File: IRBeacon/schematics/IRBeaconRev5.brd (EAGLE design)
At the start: 90 x 14.8 mm, 14 parts, among them IC1 LD117AS33TR, SW1 416131160808, X1 53048-06

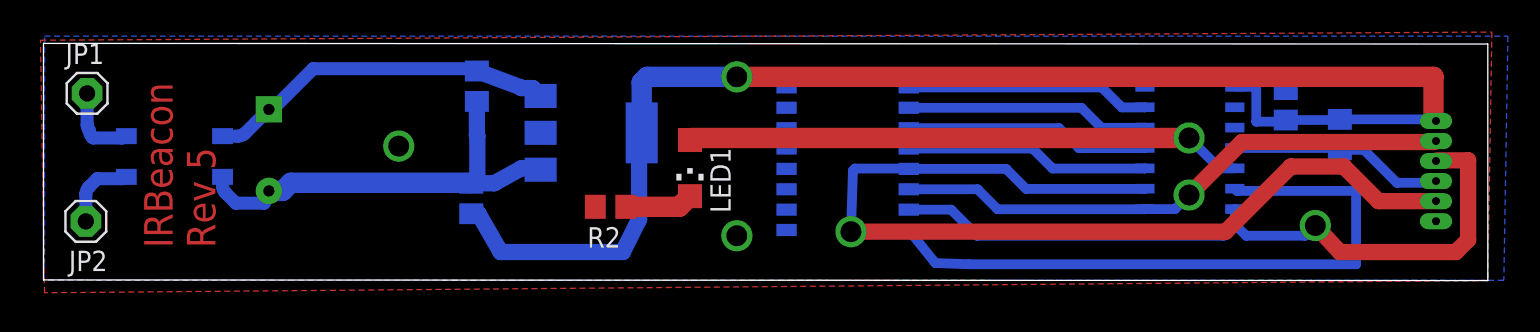
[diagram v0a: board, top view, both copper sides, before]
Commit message: More pinne fix and circuit stuff
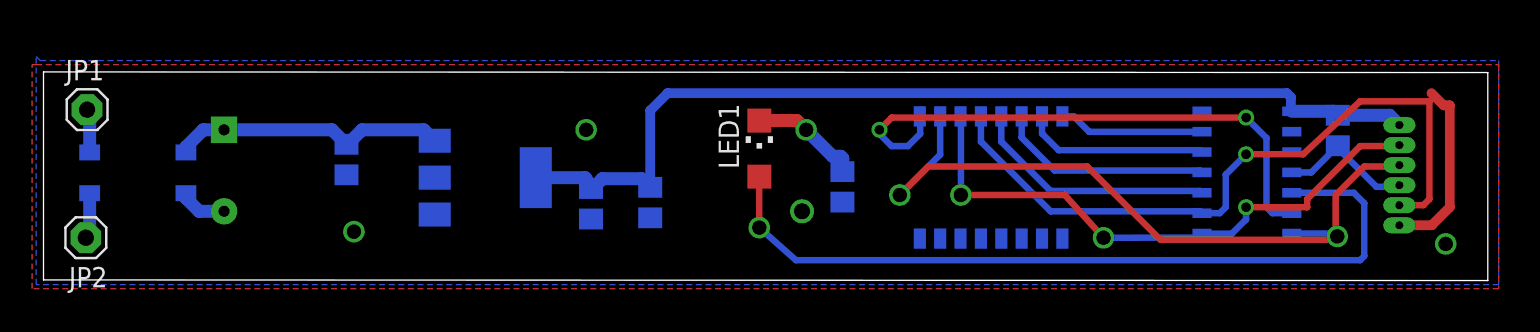
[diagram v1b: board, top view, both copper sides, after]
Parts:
- moved C1 40.1 mm to (37.8, 4.86), turned to 270 degrees
- moved R2 14.5 mm to (49.8, 5.84), flipped to the bottom, turned to 270 degrees
- moved SW1 13.8 mm to (63.5, 6.43), turned to 0 degrees
- moved C3 9.33 mm to (18.8, 7.54)
- moved C2 7.47 mm to (34.1, 4.79), turned to 270 degrees
- moved IC1 7.17 mm to (27.5, 6.42)
- moved LED1 4.49 mm to (44.6, 8.23), turned to 0 degrees
- moved U$1 3.87 mm to (75.0, 6.74)
- moved C4 3.07 mm to (11.2, 6.86)
- moved B1 2.50 mm to (5.83, 6.72)
- moved X1 2.30 mm to (85.7, 6.57)
- moved JP1 1.02 mm to (2.67, 10.7)
- moved JP2 1.02 mm to (2.59, 2.67)
- moved R1 0.28 mm to (80.6, 9.35)
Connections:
- removed net N$16: SW1.16, U$1.6
- removed net N$9: SW1.9, U$1.13
- new net N$11: SW1.9, U$1.6
- new net N$14: SW1.11, U$1.8, X1.2
- net N$10: now also SW1.10; no longer SW1.15
- net N$12: now also SW1.16, U$1.13; no longer SW1.14, U$1.8, X1.2
- net N$4: now also SW1.15, U$1.12; no longer SW1.12, U$1.10
- net N$5: now also SW1.14; no longer SW1.11
- net N$6: now also SW1.13, U$1.10; no longer SW1.10, U$1.12
- net N$8: now also SW1.12; no longer SW1.13
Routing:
- net N$16: track 41.1 -> 0.00 mm
- net N$14: track 0.00 -> 36.6 mm, vias 0 -> 3
- net N$11: track 0.00 -> 35.6 mm, vias 0 -> 2
- net VCC: track 89.3 -> 61.3 mm, vias 1 -> 0
- net N$12: track 35.2 -> 9.11 mm, vias 1 -> 0
- net N$8: track 61.7 -> 43.9 mm
- net N$9: track 15.2 -> 0.00 mm
- net N$7: track 34.8 -> 49.9 mm
- net GND: track 27.3 -> 14.4 mm, vias 2 -> 4
- net N$1: track 13.5 -> 8.59 mm
- net N$3: track 22.0 -> 17.3 mm
- net N$4: track 15.2 -> 11.5 mm
- net N$13: track 4.28 -> 7.02 mm, vias 0 -> 1
- net RAIL_A: track 4.96 -> 2.73 mm
- net N$2: track 4.75 -> 2.87 mm
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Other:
- board size 90 x 14.8 mm -> 90 x 13 mm
- board text removed: "IRBeacon Rev 5"
